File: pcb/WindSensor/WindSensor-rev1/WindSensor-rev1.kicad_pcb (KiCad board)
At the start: 2 copper layers, 20 x 20 mm, 8 parts

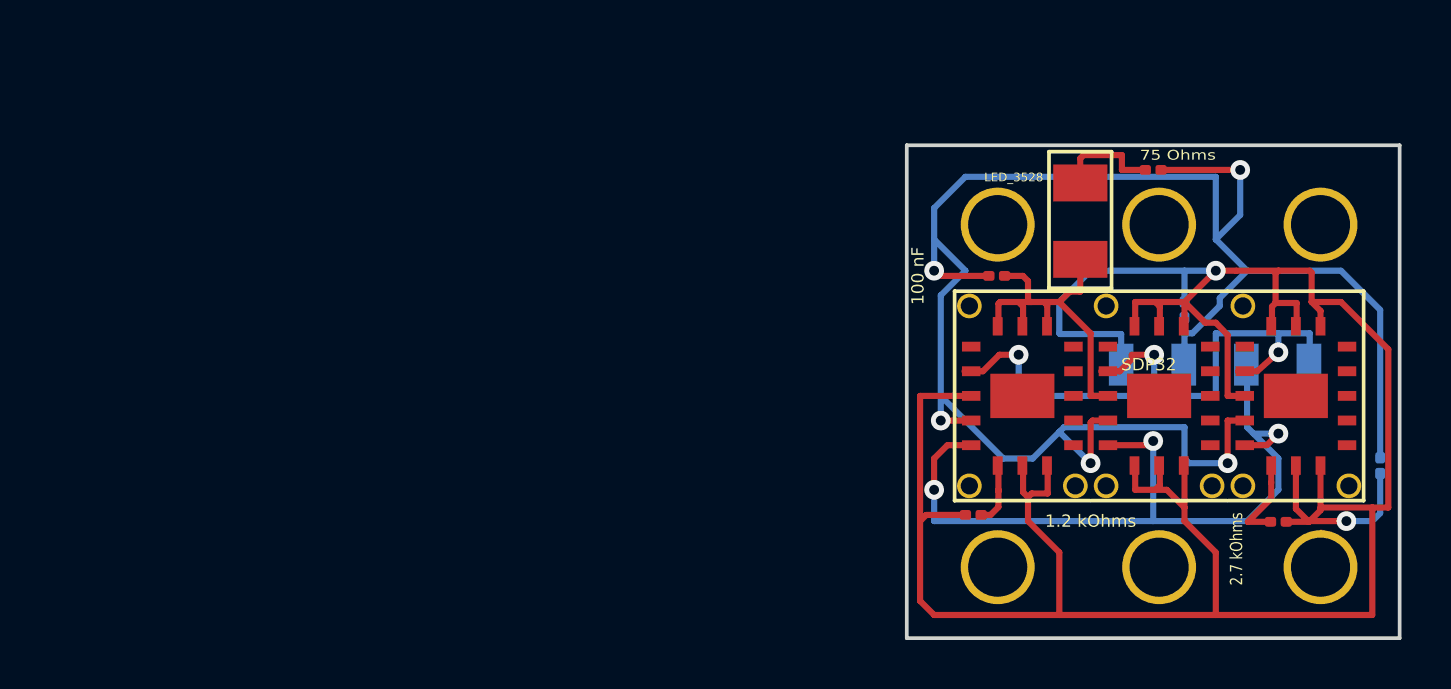
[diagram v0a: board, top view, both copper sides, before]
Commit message: getting there
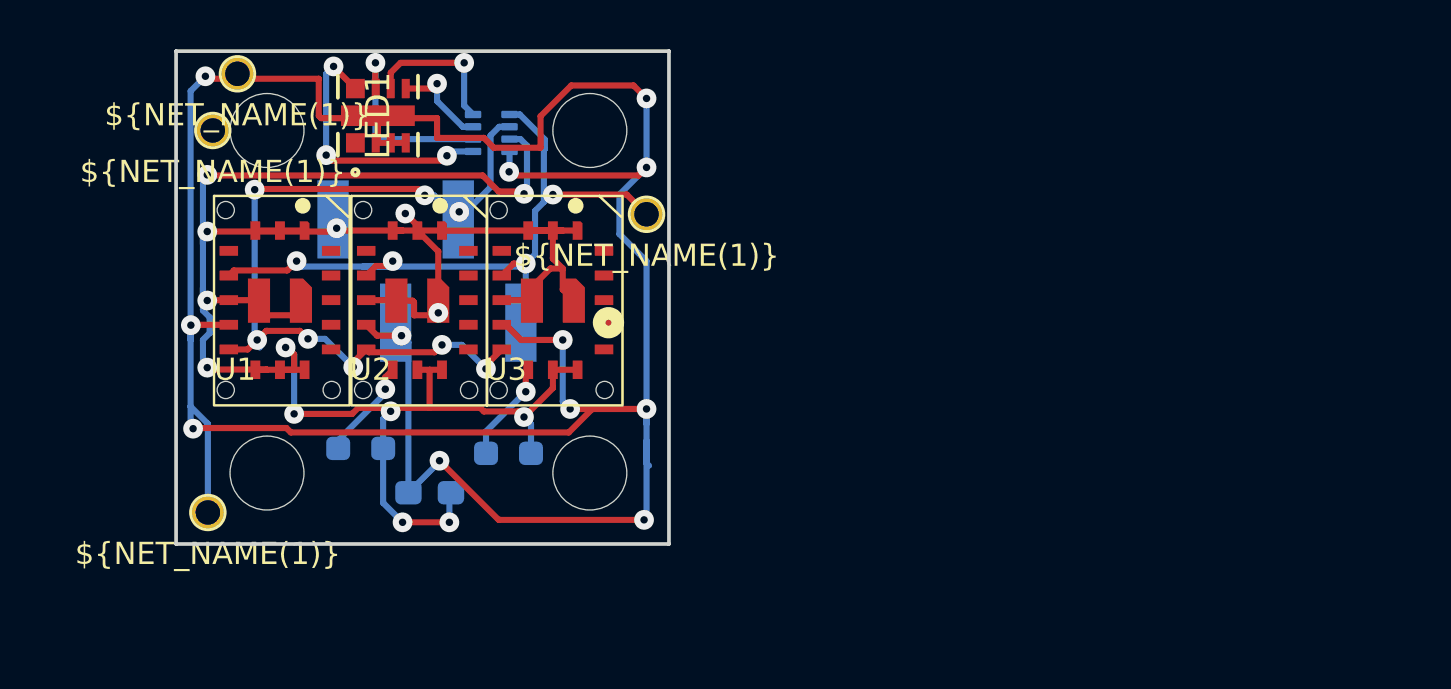
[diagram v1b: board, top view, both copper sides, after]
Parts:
- removed 1.2 kOhms: R_0201_0603Metric, Resistor_SMD:R_0201_0603Metric
- removed 100 nF: C_0201_0603Metric, Capacitor_SMD:C_0201_0603Metric
- removed 2.7 kOhms: R_0201_0603Metric, Resistor_SMD:R_0201_0603Metric
- removed 75 Ohms: R_0201_0603Metric, Resistor_SMD:R_0201_0603Metric
- removed the ? at (125.7, 86.7)
- removed the ? at (133.7, 93.0)
- removed LED_3528: LED_3528, WindSensor:LED_3528
- removed SDP32: Val**, WindSensor:SDP32
- added ?: , , F.Cu at (88.5, 79.4)
- added ?: , , F.Cu at (101.6, 93.3)
- added ?: , , F.Cu at (101.6, 79.4)
- added ?: , , F.Cu at (88.5, 93.3)
- added C1: 10u, Capacitor_SMD:C_0603_1608Metric_Pad1.08x0.95mm_HandSolder, B.Cu at (95.1, 94.1)
- added J1: Conn_I2C_Molex_705450003, WindSensor:CONN_SD-74099-1000_04_MOL, B.Cu at (95.0, 85.9)
- added LED1: 599-2310-427F, WindSensor:599-2310_DIA, F.Cu at (93.0, 78.8)
- added R1: 1.2k, Resistor_SMD:R_0603_1608Metric_Pad0.98x0.95mm_HandSolder, B.Cu at (92.3, 92.3)
- added R2: 2.7k, Resistor_SMD:R_0603_1608Metric_Pad0.98x0.95mm_HandSolder, B.Cu at (98.3, 92.5)
- added TP1: TestPoint_Probe_autonamed, argo:TestPoint_scope_probe_autonamed, F.Cu at (87.3, 77.1)
- added TP2: TestPoint_Probe_autonamed, argo:TestPoint_scope_probe_autonamed, F.Cu at (86.1, 94.9)
- added TP3: TestPoint_Probe_autonamed, argo:TestPoint_scope_probe_autonamed, F.Cu at (103.9, 82.8)
- added TP4: TestPoint_Probe_autonamed, argo:TestPoint_scope_probe_autonamed, F.Cu at (86.3, 79.4)
- added U1: SDP320x21, WindSensor:SDP32, F.Cu at (86.3, 90.6)
- added U2: SDP320x22, WindSensor:SDP32, F.Cu at (91.9, 90.6)
- added U3: SDP320x23, WindSensor:SDP32, F.Cu at (97.4, 90.6)
- added U4: LP5814DRLR, WindSensor:IC_LP5814DRLR, B.Cu at (97.6, 79.5)
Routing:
- net (no net): track 277.1 -> 0.00 mm, vias 13 -> 0
- net VDD: track 0.00 -> 117.3 mm, vias 0 -> 12
- net GND: track 0.00 -> 99.1 mm, vias 0 -> 14
- net SDA: track 0.00 -> 33.9 mm, vias 0 -> 8
- net SCL: track 0.00 -> 30.0 mm, vias 0 -> 4
- net /W: track 0.00 -> 11.2 mm, vias 0 -> 3
- net /B: track 0.00 -> 8.07 mm, vias 0 -> 1
- net /R: track 0.00 -> 6.03 mm, vias 0 -> 1
- net Net-(U2-ADDR): track 0.00 -> 4.11 mm, vias 0 -> 1
- net Net-(U3-ADDR): track 0.00 -> 4.10 mm, vias 0 -> 1
- net /G: track 0.00 -> 3.95 mm, vias 0 -> 1
